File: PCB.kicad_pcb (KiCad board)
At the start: 2 copper layers, 89 x 156.5 mm, 48 parts, among them U1 WeMos_D1_mini

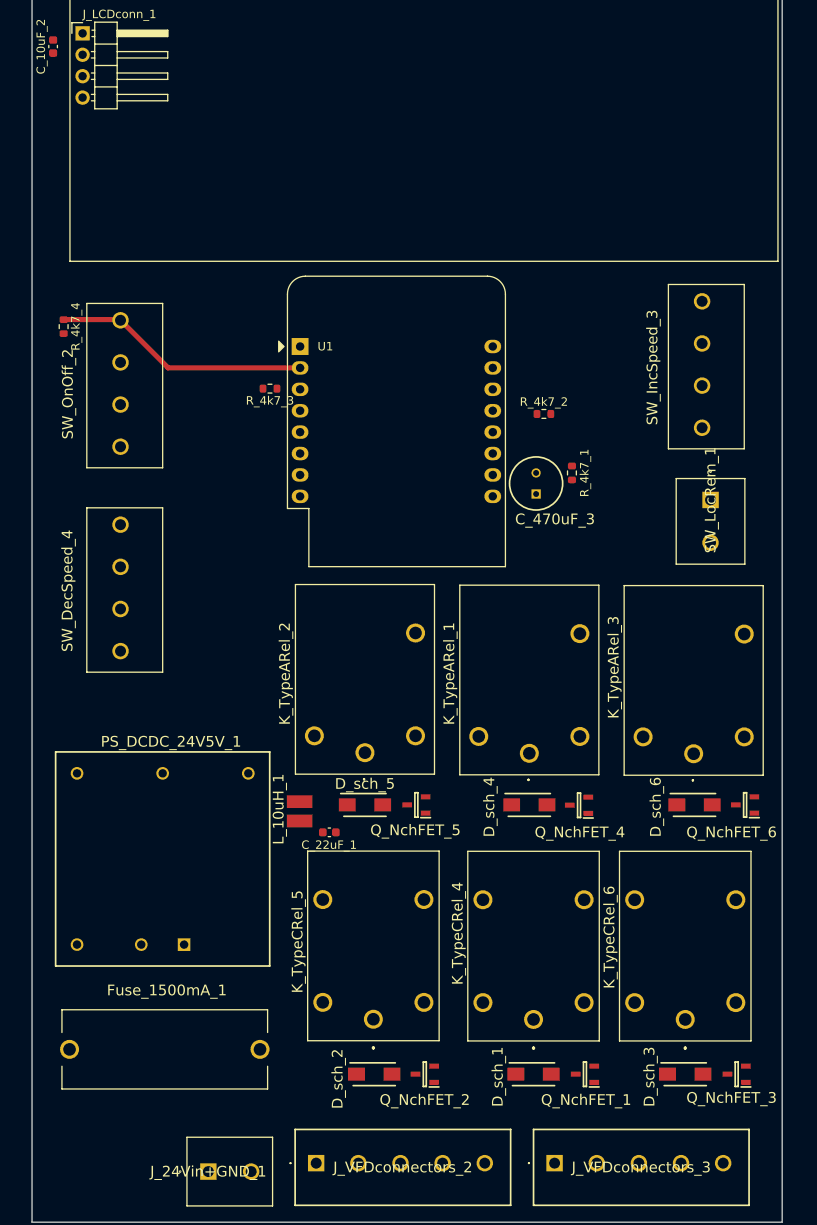
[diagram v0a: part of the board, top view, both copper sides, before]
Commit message: zacal jsem wirovat draty a via
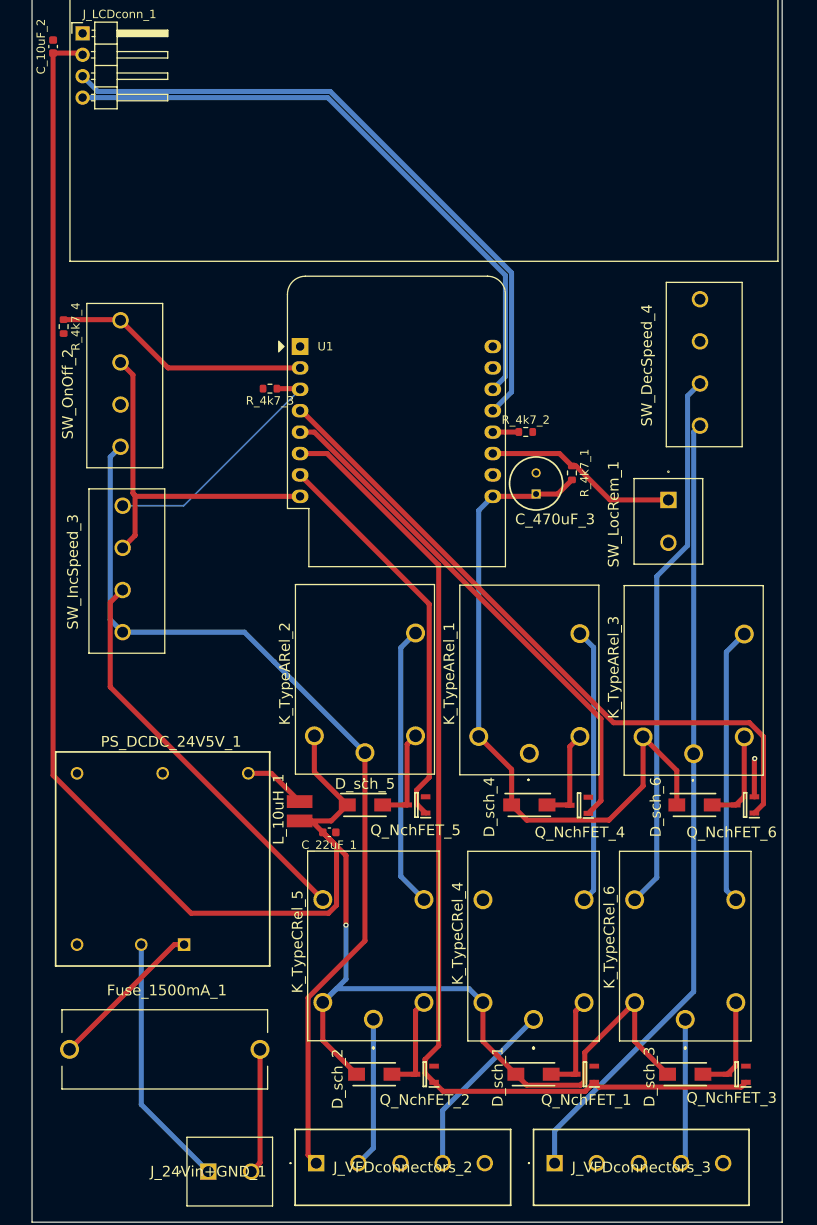
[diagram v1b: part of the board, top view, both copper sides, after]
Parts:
- moved SW_DecSpeed_4 73.8 mm to (138.8, 127.0)
- moved SW_IncSpeed_3 72.9 mm to (70.2, 151.5)
- moved SW_LocRem_1 5.00 mm to (135.0, 135.8)
- moved R_4k7_2 3.04 mm to (118.1, 127.8)
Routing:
- net VCC: track 0.00 -> 335.5 mm, vias 0 -> 1
- net DO7: track 0.00 -> 122.8 mm
- net J3 24V: track 0.00 -> 109.7 mm
- net J4 24V: track 0.00 -> 94.6 mm
- net DO5: track 0.00 -> 80.5 mm
- net SDA: track 0.00 -> 77.8 mm
- net SCL: track 0.00 -> 73.0 mm
- net local DI2: track 0.00 -> 64.5 mm
- net DO6: track 0.00 -> 61.6 mm
- net local DI1: track 0.00 -> 47.8 mm
- net DO8: track 0.00 -> 47.5 mm
- net MCU 3V3: track 0.00 -> 43.0 mm
- net remote DI1: track 0.00 -> 33.5 mm
- net remote DI2: track 0.00 -> 32.9 mm
- net remote DI0: track 0.00 -> 32.7 mm
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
